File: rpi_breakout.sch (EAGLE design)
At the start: 29 parts, among them U2 TXB0108, U3 TXB0108

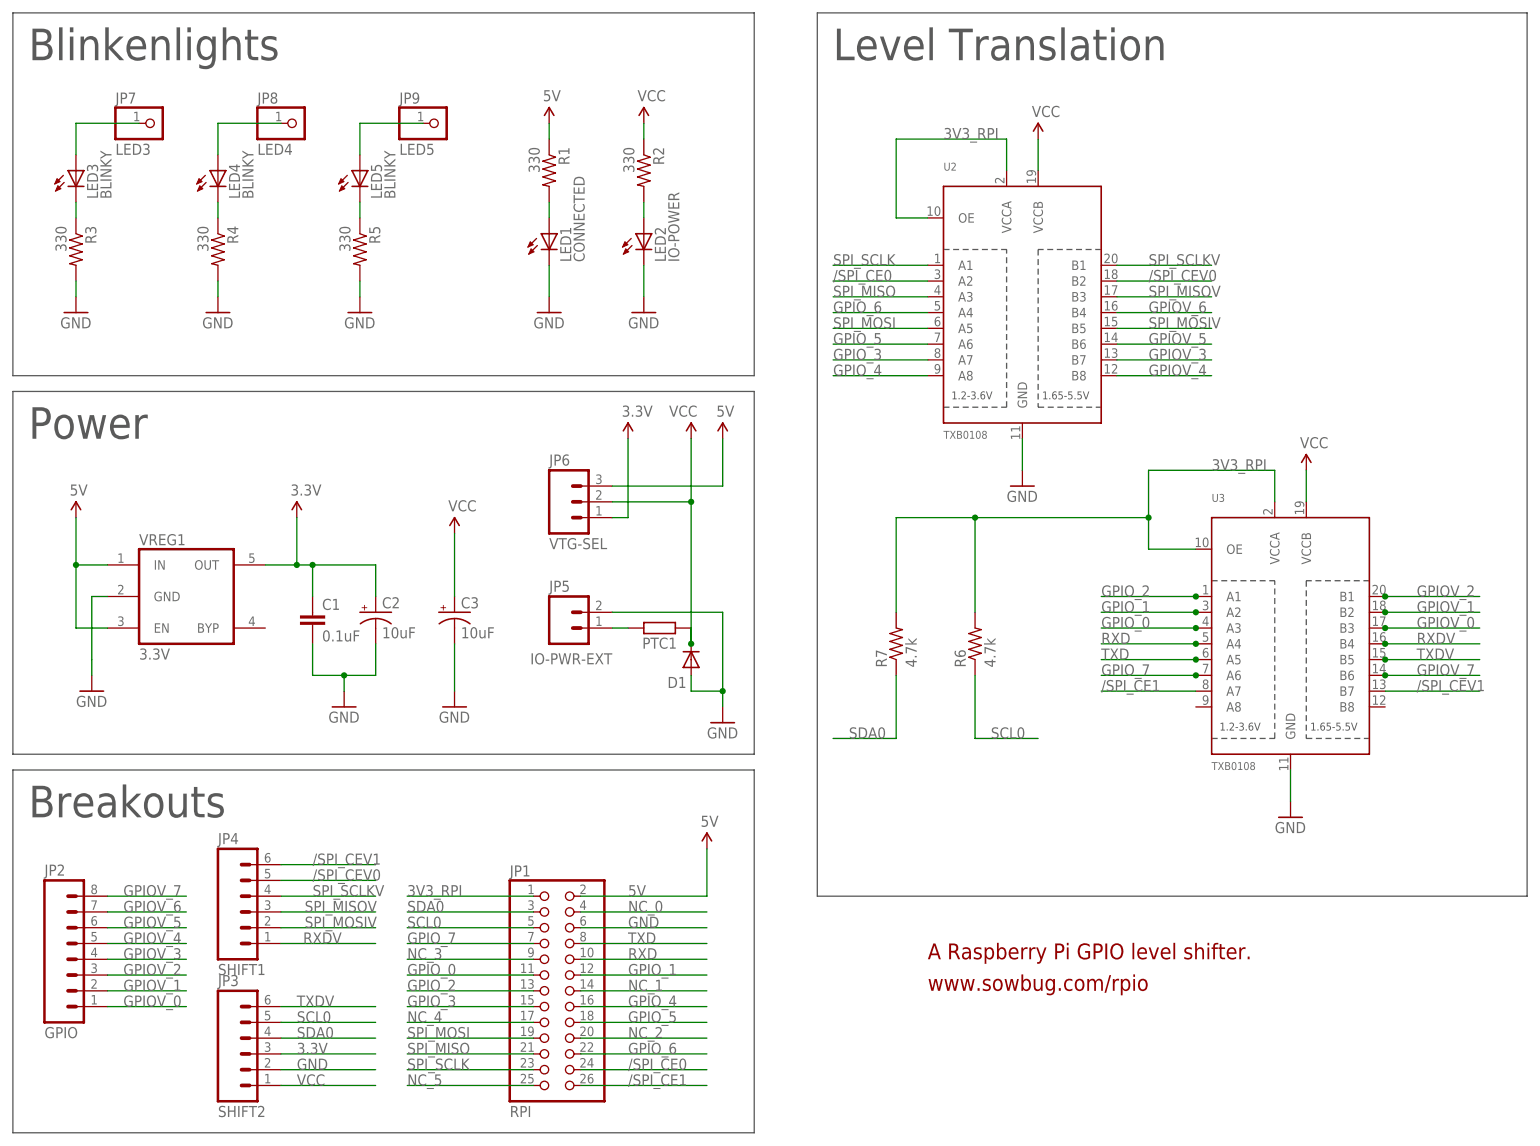
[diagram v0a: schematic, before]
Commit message: Interim checkin. Autorouter is SLOW today.
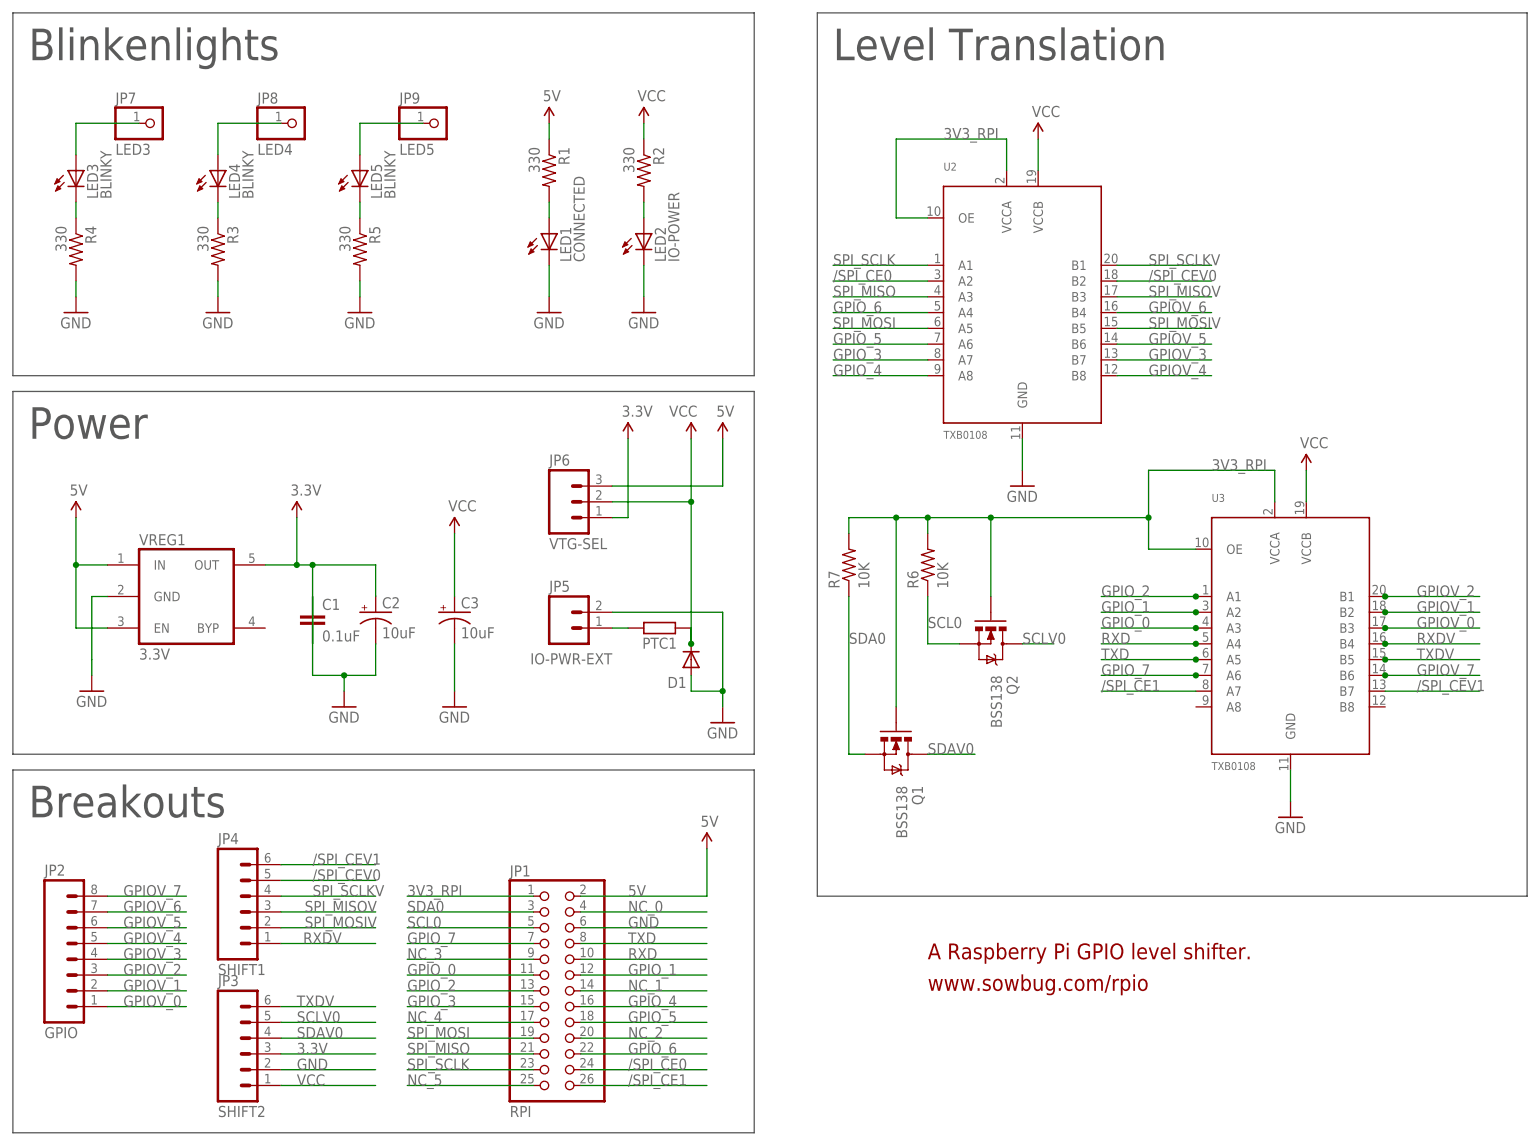
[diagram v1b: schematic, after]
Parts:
- added Q1, Q2: BSS138, rpi_breakout:SPARKFUN_MOSFET-NCHANNELSMD
- C1: device SparkFun:CAP0805 -> rpi_breakout:SPARKFUN_CAP0805
- C2, C3: device SparkFun:CAP_POL1206 -> rpi_breakout:SPARKFUN_CAP_POL1206
- D1: device SparkFun-DiscreteSemi:DIODESOD -> rpi_breakout:SPARKFUN-DISCRETESEMI_DIODESOD
- JP1: device pinhead:PINHD-2X13 -> rpi_breakout:PINHEAD_PINHD-2X13
- JP2: device SparkFun:M08LOCK -> rpi_breakout:SPARKFUN_M08LOCK
- JP3, JP4: device SparkFun:M06FEMALE_LOCK -> rpi_breakout:SPARKFUN_M06LOCK
- JP5: device SparkFun:M02PTH -> rpi_breakout:SPARKFUN_M02LOCK
- JP6: device SparkFun:M03PTH -> rpi_breakout:SPARKFUN_M03LOCK
- JP7, JP8, JP9: device adafruit:PINHD-1X1CB -> rpi_breakout:ADAFRUIT_PINHD-1X1
- LED1, LED2, LED3, LED4, LED5: device adafruit:LEDCHIPLED_0805 -> rpi_breakout:PROGRAMMER_SPARKFUN_LED
- PTC1: device rcl:R-EU_R1206 -> rpi_breakout:RCL_R-EU_R1206
- R1, R2, R3, R4, R5: device SparkFun:RESISTOR0805-RES -> rpi_breakout:SPARKFUN_RESISTOR0805-RES
- R6, R7: value 4.7k -> 10K; device rcl:R-US_0207/10 -> rpi_breakout:SPARKFUN_RESISTOR0805-RES
- U2, U3: device rpi_breakout:TXB0108PWR -> rpi_breakout:RPI_BREAKOUT_TXB0108PWR
- VREG1: device dp_devices:IC_VREG_5PINS-SOT-23-5 -> rpi_breakout:DP_DEVICES_IC_VREG_5PINS-SOT-23-5
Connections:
- new net SCLV0: JP3.5, Q2.D
- new net SDAV0: JP3.4, Q1.D
- net 3.3V: now also C1.2; no longer C1.1
- net 3V3_RPI: now also Q1.G, Q2.G
- net GND: now also C1.1; no longer C1.2
- net N$3: now also R4.1; no longer R3.1
- net N$4: now also R3.1; no longer R4.1
- net SCL0: now also Q2.S; no longer JP3.5
- net SDA0: now also Q1.S; no longer JP3.4
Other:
- moved on the sheet: R3, R4, R6, R7
